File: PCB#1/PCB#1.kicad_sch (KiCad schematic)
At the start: 33 parts, among them J2 Conn_01x02, J3 Conn_02x18_Odd_Even, J4 Conn_02x18_Odd_Even, P1 USB_C_Plug_USB2.0, U1 RP2040, U2 ICM-20948, U3 NCP1117-3.3_SOT223, U4 W25Q128JVS, U5 NCP1117-1.8_SOT223, Y1 Crystal_GND24

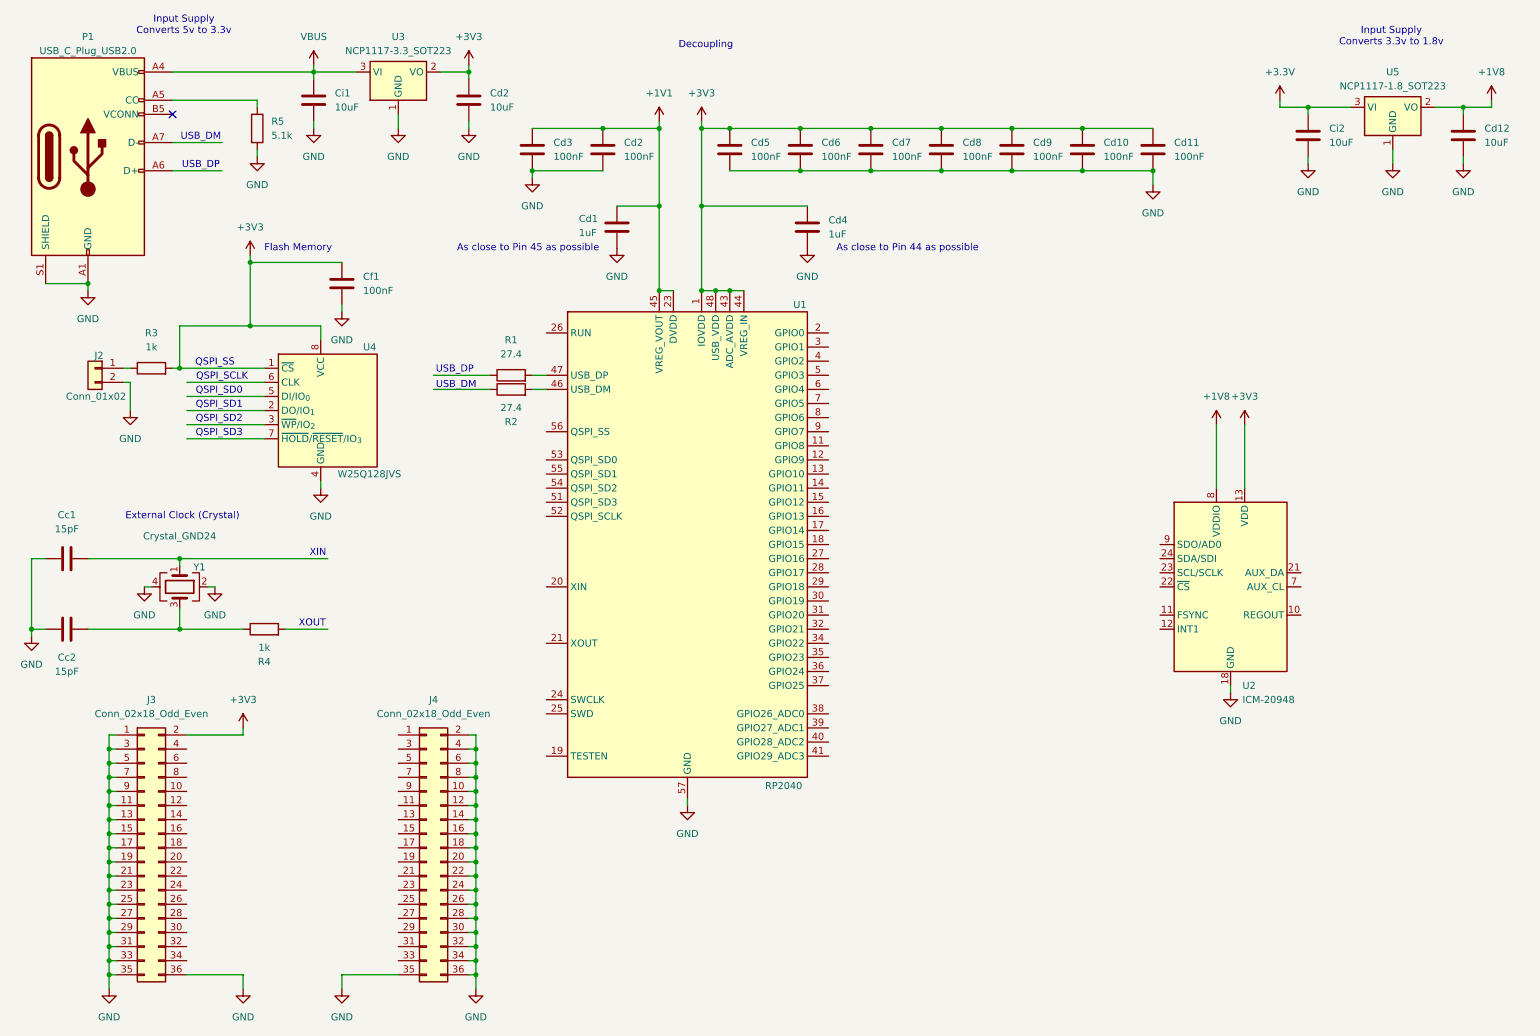
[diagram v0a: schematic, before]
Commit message: Add files via upload
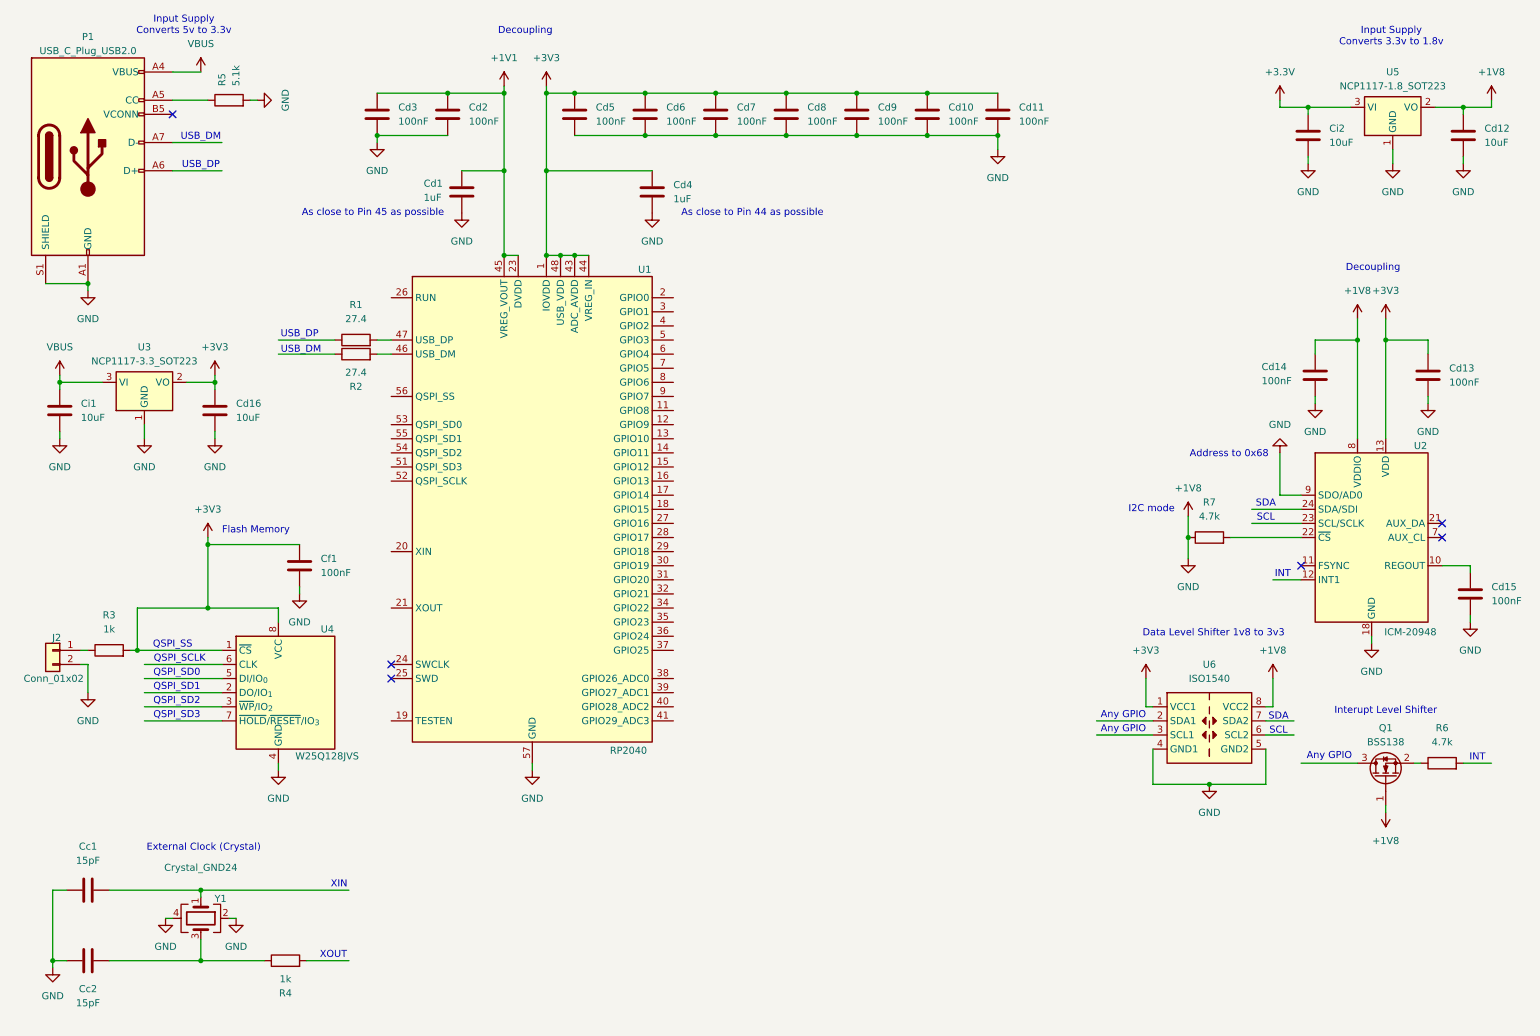
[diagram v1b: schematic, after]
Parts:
- removed Cd2: 10uF, symbol Device:C
- removed J3, J4: Conn_02x18_Odd_Even, symbol Connector_Generic:Conn_02x18_Odd_Even
- added Cd13, Cd14, Cd15: 100nF, symbol Device:C
- added Cd16: 10uF, symbol Device:C
- added Q1: BSS138, Package_TO_SOT_SMD:SOT-23, symbol Transistor_FET:BSS138
- added R6, R7: 4.7k, symbol Device:R
- added U6: ISO1540, Package_SO:SOIC-8_3.9x4.9mm_P1.27mm, symbol Isolator:ISO1540
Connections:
- net GND is gone; now on net +1V8: Cc1.2, Cc2.2, Cd1.2, Cd10.2, Cd11.2, Cd12.2, Cd2.2, Cd3.2, Cd4.2, Cd5.2, Cd6.2, Cd7.2, Cd8.2, Cd9.2, Cf1.2, Ci1.2, Ci2.2, J2.2 (Pin_2), P1.A1 (GND), P1.A12 (GND), P1.B1 (GND), P1.B12 (GND), P1.S1 (SHIELD), R5.2, U1.57 (GND), U2.18 (GND), U2.20 (GND), U3.1 (GND), U4.4 (GND), U5.1 (GND), Y1.2, Y1.4
- net +1V8: now also U2.9 (SDO/AD0), Cd13.2, Cd14.1, Cd14.2, Cd15.2, Cd16.2, Q1.1 (G), R7.1, U6.4 (GND1), U6.5 (GND2), U6.8 (VCC2)
- net +3V3: now also Cd13.1, Cd16.1, U6.1 (VCC1)
- net at U2.10 (REGOUT): now also Cd15.1
- net at U2.22 (~{CS}): now also R7.2
- new net: Q1.2 (S), R6.1
- no-connect marks 1 -> 6
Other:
- note added: "Address to 0x68"
- note added: "Any GPIO"
- note added: "Data Level Shifter 1v8 to 3v3"
- note added: "I2C mode"
- note added: "INT"
- note added: "Interupt Level Shifter"
- note added: "SCL"
- note added: "SDA"
- moved on the sheet: Cc1, Cc2, Cd1, Cd10, Cd11, Cd2, Cd3, Cd4, Cd5, Cd6, Cd7, Cd8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
